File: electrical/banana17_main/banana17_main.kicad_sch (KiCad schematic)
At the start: 28 parts, among them J1 USB_C_Receptacle_USB2.0_16P, U1 RP2040, U2 NCP1117-3.3_SOT223, U3 ssd1306_128x32, U4 W25Q128JVS, Y1 ABMB-272-T3

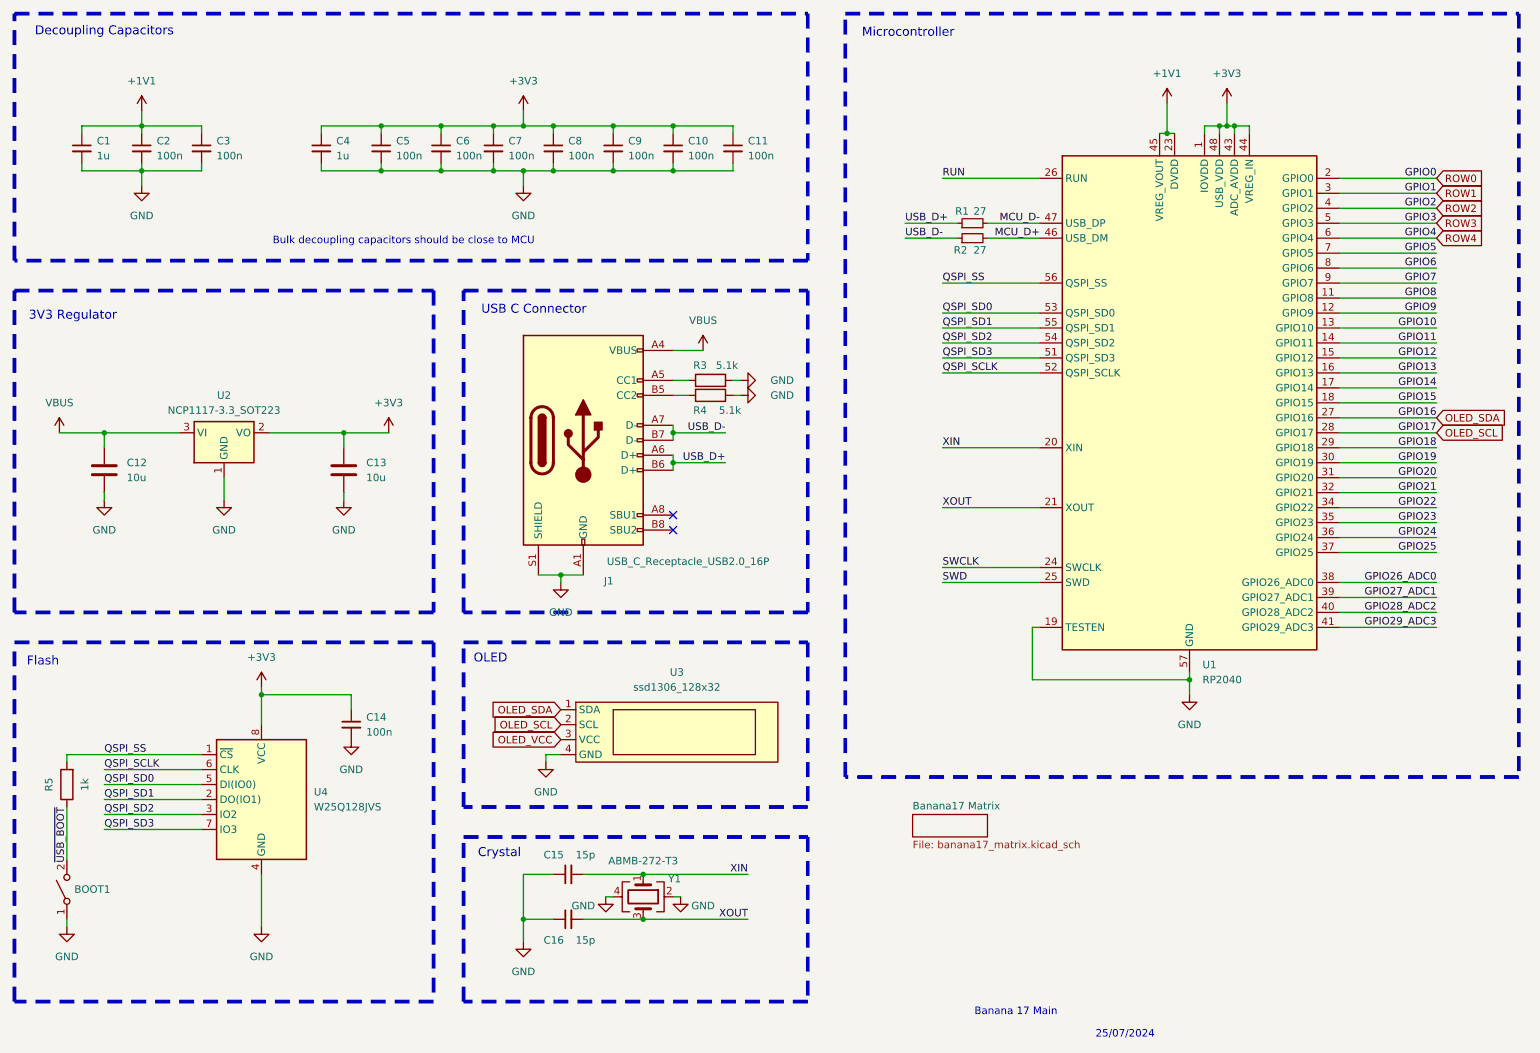
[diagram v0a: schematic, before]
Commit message: Initial PCB complete.
Initial PCB complete.
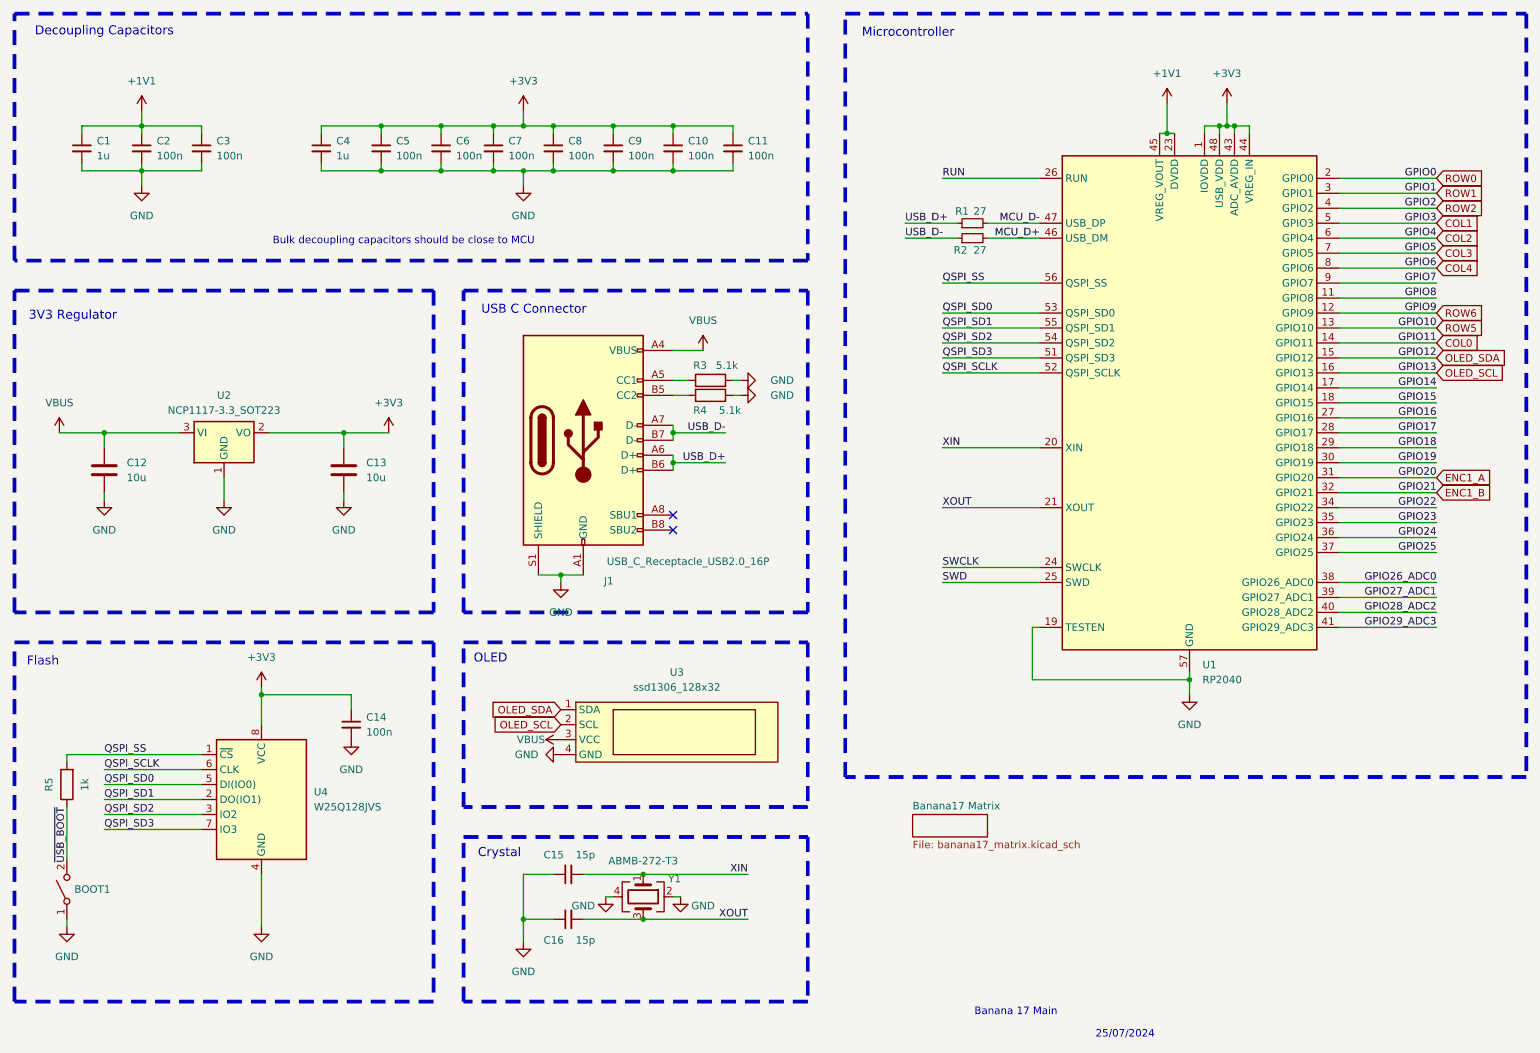
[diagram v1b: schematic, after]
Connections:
- net GPIO12 is gone; now on net OLED_SDA: U1.15 (GPIO12)
- net GPIO13 is gone; now on net OLED_SCL: U1.16 (GPIO13)
- net OLED_VCC is gone; now on net VBUS: U3.3 (VCC)
- net OLED_SCL: no longer U1.28 (GPIO17)
- net OLED_SDA: no longer U1.27 (GPIO16)
- net GPIO10 renamed ROW5
- net GPIO11 renamed COL0
- net GPIO20 renamed ENC1_A
- net GPIO21 renamed ENC1_B
- net GPIO5 renamed COL3
- net GPIO6 renamed COL4
- net GPIO9 renamed ROW6
- net ROW3 renamed COL1
- net ROW4 renamed COL2
- new net GPIO16: U1.27 (GPIO16)
- new net GPIO17: U1.28 (GPIO17)
